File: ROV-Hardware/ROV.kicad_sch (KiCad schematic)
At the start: 18 parts, among them J1 Screw_Terminal_01x02, J2 Screw_Terminal_01x02, J3 Screw_Terminal_01x04, SW1 SW_Wuerth_450301014042, U1 LM7812_TO220, U2 LM7805_TO220, U3 ESP32-S3-DEVKITC-1-N8R2, U4 MPU6050, U5 ZK-BM!, U6 ZK-BM!, U7 ZK-BM!

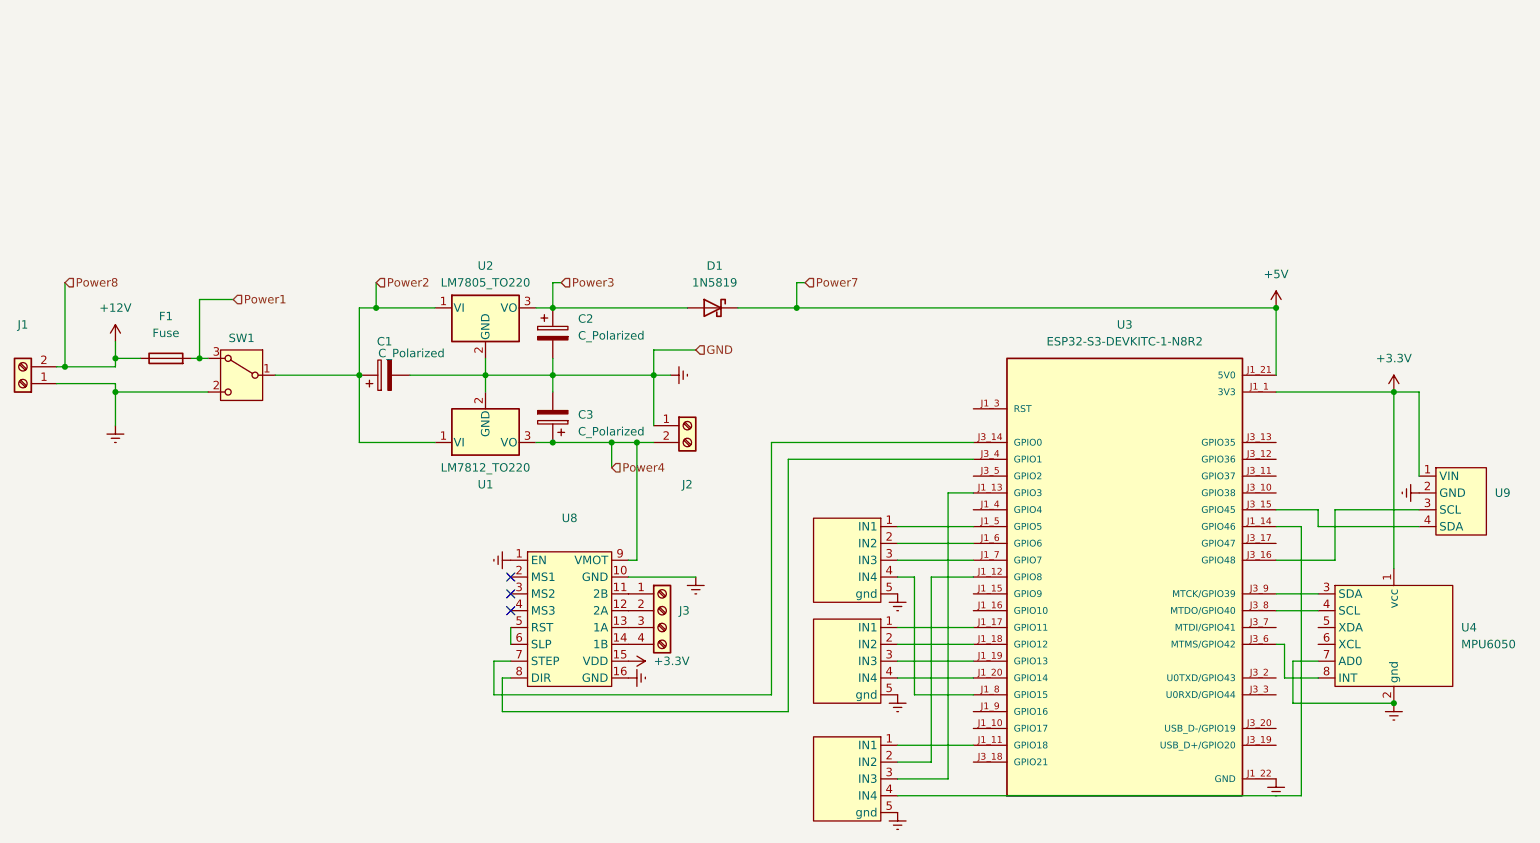
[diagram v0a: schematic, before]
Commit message: refresh
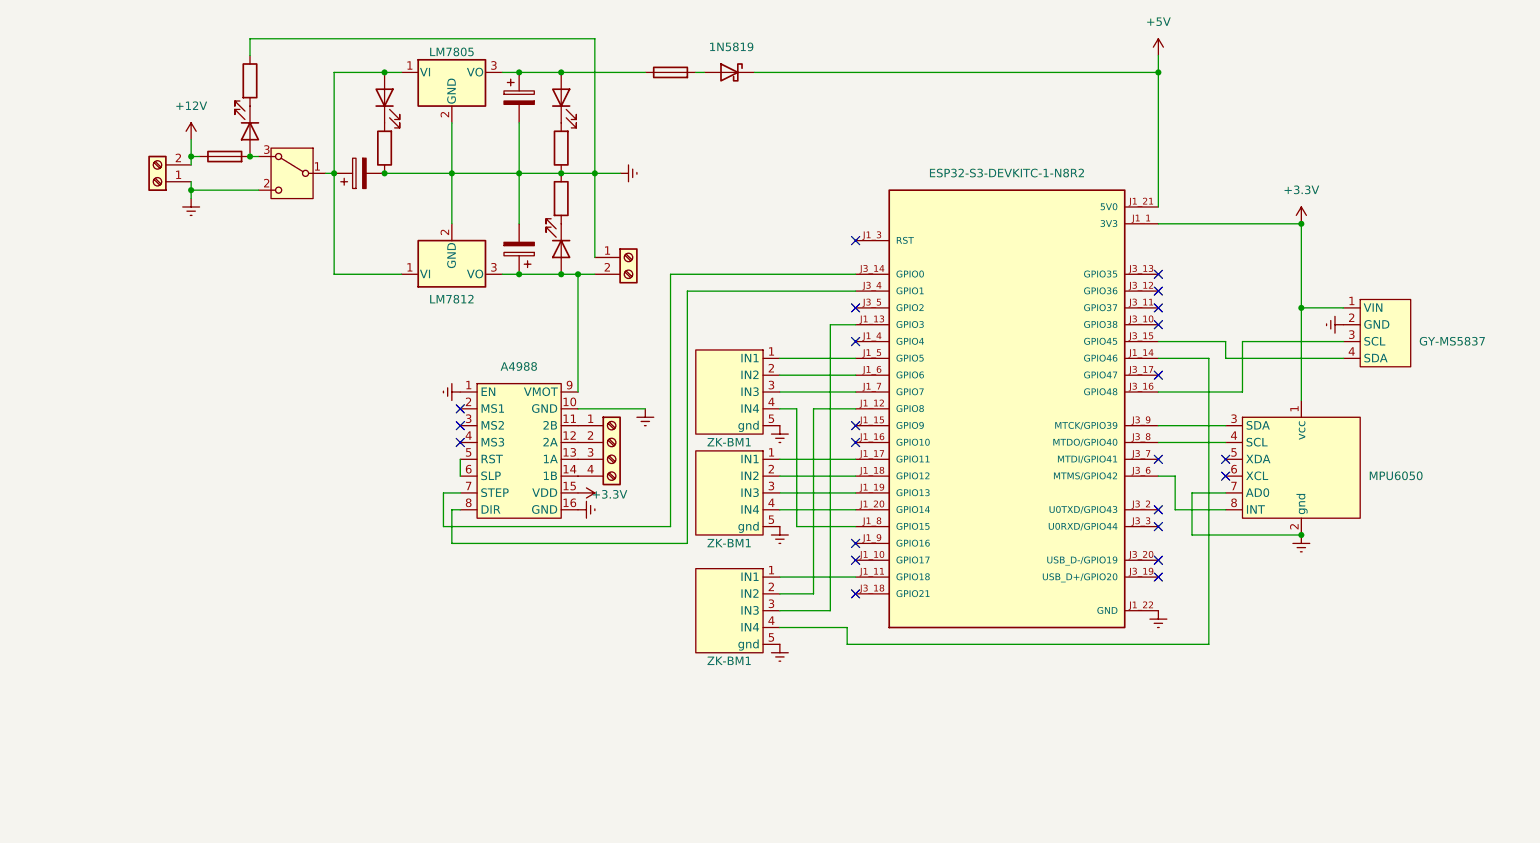
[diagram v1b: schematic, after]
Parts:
- added D2, D3, D4, D5: LED, LED_THT:LED_D3.0mm, symbol Device:LED
- added F2: fuse, Fuse:Fuseholder_Clip-5x20mm_Schurter_CQM_Inline_P20.60x5.00mm_D1.00mm_Horizontal, symbol Device:Fuse
- added R1, R2, R3, R4: R, Resistor_THT:R_Axial_DIN0204_L3.6mm_D1.6mm_P5.08mm_Horizontal, symbol Device:R
- C1, C2, C3: value C_Polarized -> capacitor
- F1: value Fuse -> fuse
- J1: value Screw_Terminal_01x02 -> T-block; footprint TerminalBlock:TerminalBlock_MaiXu_MX126-5.0-02P_1x02_P5.00mm -> Connector_AMASS:AMASS_XT60-F_1x02_P7.20mm_Vertical
- J2: value Screw_Terminal_01x02 -> T-block
- SW1: value SW_Wuerth_450301014042 -> switch
- U1: value LM7812_TO220 -> LM7812
- U2: value LM7805_TO220 -> LM7805
- U5, U6, U7: value ZK-BM! -> ZK-BM1
- U8: value ~ -> A4988
- U9: value ~ -> GY-MS5837
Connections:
- net GND: now also R1.1, R2.1, R3.1, R4.1
- net Power1: no longer names the net of F1.2, SW1.3 (A)
- net Power1: now also D5.2 (A)
- net Power2: no longer names the net of C1.1, SW1.1 (B), U1.1 (VI), U2.1 (VI)
- net Power2: now also D2.2 (A)
- net Power3: no longer names the net of C2.1, U2.3 (VO)
- net Power3: now also D3.2 (A), F2.1; no longer D1.2 (A)
- net Power4: no longer names the net of C3.1, J2.2 (Pin_2), U1.3 (VO), U8.9 (VMOT)
- net Power4: now also D4.2 (A)
- new net: D2.1 (K), R1.2
- new net: D5.1 (K), R4.2
- new net: D4.1 (K), R3.2
- new net: D3.1 (K), R2.2
- new net: D1.2 (A), F2.2
- no-connect marks 3 -> 23
